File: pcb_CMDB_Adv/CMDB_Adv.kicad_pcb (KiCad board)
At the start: 6 copper layers, 59.7 x 78 mm, 9 parts, among them J1 POWER TERMINAL, J12 CONN_USB3_A, J13 CONN_USB_PWR_OTG, J15 CONN_DOCK, J16 CONN_CAM1, J17 CONN_CAM0, J2 Bus_M.2_Socket_M, J4 J_PSU_EN

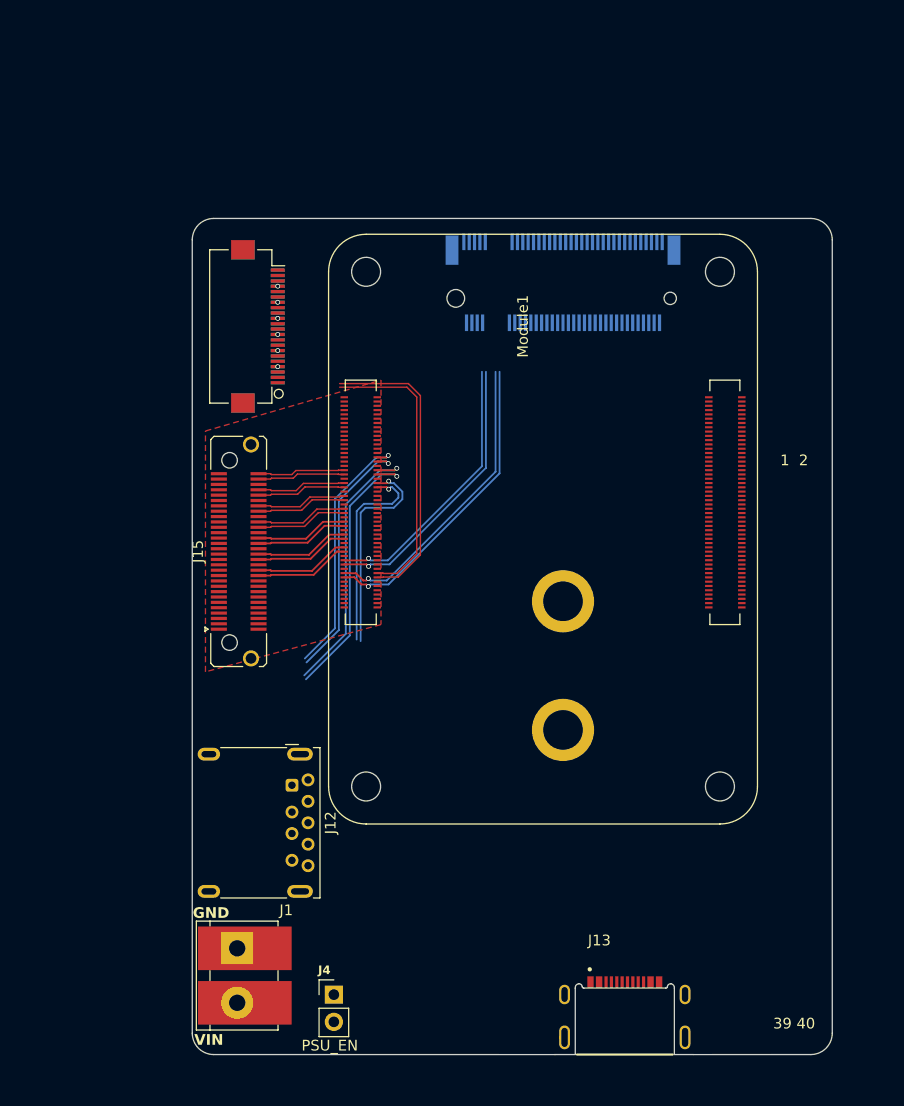
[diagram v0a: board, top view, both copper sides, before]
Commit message: CMDB-Adv PCB WIP
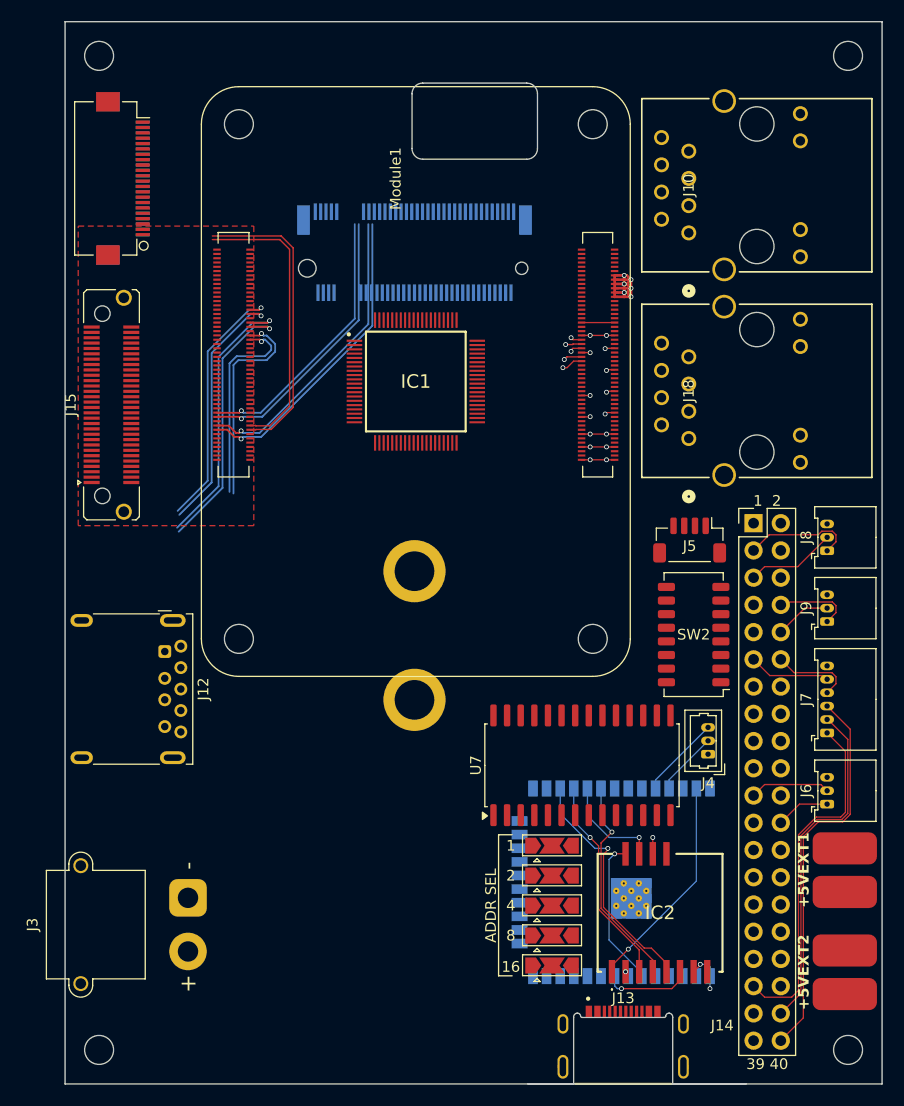
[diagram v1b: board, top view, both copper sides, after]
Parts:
- removed J1: POWER TERMINAL, CMDB_Adv:Power Terminal
- added H1: MountingHole, CMDB_Adv:MountingHole_2.7mm_M2.5_DIN965, F.Cu at (137.6, 53.4)
- added H2: MountingHole, CMDB_Adv:MountingHole_2.7mm_M2.5_DIN965, F.Cu at (207.4, 53.4)
- added H3: MountingHole, CMDB_Adv:MountingHole_2.7mm_M2.5_DIN965, F.Cu at (207.4, 146.1)
- added H4: MountingHole, CMDB_Adv:MountingHole_2.7mm_M2.5_DIN965, F.Cu at (137.6, 146.1)
- added IC1: KSZ8795CLXCC, CMDB_Adv:QFP40P1200X1200X160-80N, F.Cu at (167.1, 83.7)
- added IC2: Wio-SX1262, CMDB_Adv:Wio-SX1262, F.Cu at (189.9, 133.3)
- added J10: ETH1, CMDB_Adv:CONN12_ARJM11B1-009-AB-EW2_ABR, F.Cu at (198.9, 65.4)
- added J14: CONN_HAT, Connector_PinHeader_2.54mm:PinHeader_2x20_P2.54mm_Vertical, F.Cu at (198.6, 96.9)
- added J18: ETH2, CMDB_Adv:CONN12_ARJM11B1-009-AB-EW2_ABR, F.Cu at (198.9, 84.6)
- added J20: CONN_5VEXT1, Connector_Wire:SolderWirePad_1x01_SMD_3x6mm, F.Cu at (207.1, 131.3)
- added J21: CONN_5VEXT1_GND, Connector_Wire:SolderWirePad_1x01_SMD_3x6mm, F.Cu at (207.1, 127.3)
- added J22: CONN_5VEXT2, Connector_Wire:SolderWirePad_1x01_SMD_3x6mm, F.Cu at (207.1, 140.9)
- added J23: CONN_5VEXT2_GND, Connector_Wire:SolderWirePad_1x01_SMD_3x6mm, F.Cu at (207.1, 136.8)
- added J3: CONN_VIN, Connector_AMASS:AMASS_XT30PW-M_1x02_P2.50mm_Horizontal, F.Cu at (145.9, 131.9)
- added J5: CONN_FAN, Connector_JST:JST_SH_BM04B-SRSS-TB_1x04-1MP_P1.00mm_Vertical, F.Cu at (192.7, 98.5)
- added J6: CONN_UART3, Connector_Molex:Molex_PicoBlade_53048-0310_1x03_P1.25mm_Horizontal, F.Cu at (205.5, 123.1)
- added J7: CONN_SPI, Connector_Molex:Molex_PicoBlade_53048-0610_1x06_P1.25mm_Horizontal, F.Cu at (205.5, 116.5)
- added J8: CONN_I2C, Connector_Molex:Molex_PicoBlade_53048-0310_1x03_P1.25mm_Horizontal, F.Cu at (205.5, 99.5)
- added J9: CONN_UART0, Connector_Molex:Molex_PicoBlade_53048-0310_1x03_P1.25mm_Horizontal, F.Cu at (205.5, 106.1)
- added JP10: ADDR16, Jumper:SolderJumper-3_P2.0mm_Open_TrianglePad1.0x1.5mm, F.Cu at (179.8, 138.2)
- added JP6: ADDR1, Jumper:SolderJumper-3_P2.0mm_Open_TrianglePad1.0x1.5mm, F.Cu at (179.8, 127.0)
- added JP7: ADDR2, Jumper:SolderJumper-3_P2.0mm_Open_TrianglePad1.0x1.5mm, F.Cu at (179.8, 129.8)
- added JP8: ADDR4, Jumper:SolderJumper-3_P2.0mm_Open_TrianglePad1.0x1.5mm, F.Cu at (179.8, 132.6)
- added JP9: ADDR8, Jumper:SolderJumper-3_P2.0mm_Open_TrianglePad1.0x1.5mm, F.Cu at (179.8, 135.4)
- added SW2: SW_CONFIG, Button_Switch_SMD:SW_DIP_SPSTx08_Slide_Copal_CHS-08A_W5.08mm_P1.27mm_JPin, F.Cu at (193.0, 107.3)
- added U5: ESP32-WROOM-32UE, RF_Module:ESP32-WROOM-32UE, B.Cu at (186.2, 130.4)
- added U7: MCP23017_SO, Package_SO:SOIC-28W_7.5x17.9mm_P1.27mm, F.Cu at (182.6, 119.5)
- J4: value J_PSU_EN -> J_ESP_DBG_UART; footprint Connector_PinHeader_2.54mm:PinHeader_1x02_P2.54mm_Vertical -> Connector_Molex:Molex_PicoBlade_53047-0310_1x03_P1.25mm_Vertical
- moved J4 41.5 mm to (194.4, 118.5), turned to 90 degrees
- moved J16 18.7 mm to (139.8, 64.8)
- moved J17 18.7 mm to (139.8, 64.8)
- moved Module1 18.2 mm to (183.6, 59.7)
- moved J15 18.1 mm to (138.8, 85.9)
- moved J12 17.2 mm to (143.7, 108.9)
- moved J2 14.1 mm to (167.0, 73.2)
- moved J13 2.74 mm to (186.5, 147.6)
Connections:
- net /CM5/+5v renamed /+5VPB
- net /CM5/VBAT renamed /CM5/+3V3STB
- net /M2_3V3 renamed /+3V3PB1
- J13 pad A6: /Connectors/USBC.D_P -> /CM5/USBC.D_P
- J13 pad A7: /Connectors/USBC.D_N -> /CM5/USBC.D_N
- J13 pad B6: /Connectors/USBC.D_P -> /CM5/USBC.D_P
- J13 pad B7: /Connectors/USBC.D_N -> /CM5/USBC.D_N
- J15 pad 1: /Connectors/+3.3v -> /Connectors/+5V
- J15 pad 10: unconnected-(J15-Pin_10-Pad10) -> GND
- J15 pad 3: /Connectors/+5v -> /Connectors/+5V
- J15 pad 4: unconnected-(J15-Pin_4-Pad4) -> /CM5/+3V3RPi
- J15 pad 5: unconnected-(J15-Pin_5-Pad5) -> /Connectors/+VBUS_USBA
- J15 pad 7: unconnected-(J15-Pin_7-Pad7) -> /Connectors/+VBUS_USBA
- J15 pad 9: unconnected-(J15-Pin_9-Pad9) -> GND
- J16 pad 22: /Connectors/+3.3v -> /CM5/+3V3RPi
- J17 pad 22: /Connectors/+3.3v -> /CM5/+3V3RPi
- J4 pad 1: /PSU/VIN -> GND
- J4 pad 2: /PSU/PSU_EN -> /Platform Controller/DBG_UART_TX
- Module1 pad 11: GND -> /CM5/ETH0.P2_P
- Module1 pad 35: GND -> /CM5/GPIO1_RAW
- Module1 pad 36: GND -> /CM5/GPIO0_RAW
- Module1 pad 4: GND -> /CM5/ETH0.P1_P
- Module1 pad 41: GND -> /CM5/GP.25
- Module1 pad 51: /CM5/GPIO15_RAW -> /CM5/GP.15
- Module1 pad 55: /CM5/GPIO14_RAW -> /CM5/GP.14
- Module1 pad 6: GND -> /CM5/ETH0.P1_N
- Module1 pad 62: GND -> /CM5/CMD
- Module1 pad 78: /CM5/+3.3v_RPi -> /CM5/+3V3RPi
- Module1 pad 84: /CM5/+3.3v_RPi -> /CM5/+3V3RPi
- Module1 pad 86: /CM5/+3.3v_RPi -> /CM5/+3V3RPi
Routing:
- net /CM5/GP.17: track 0.00 -> 50.2 mm, vias 0 -> 1
- net /CM5/GP.3: track 0.00 -> 44.5 mm, vias 0 -> 1
- net /CM5/GP.2: track 0.00 -> 43.5 mm, vias 0 -> 1
- net /Connectors/GP.27: track 0.00 -> 42.3 mm
- net /CM5/GP.22: track 0.00 -> 41.7 mm
- net /CM5/GP.4: track 0.00 -> 37.0 mm, vias 0 -> 1
- net /CM5/GP.21: track 0.00 -> 36.1 mm
- net /CM5/GP.19: track 0.00 -> 32.7 mm
- net /CM5/GP.20: track 0.00 -> 32.2 mm
- net GND: track 0.00 -> 26.7 mm, vias 6 -> 18
- net /Platform Controller/LORA_RESET: track 0.00 -> 22.6 mm, vias 0 -> 1
- net /Platform Controller/LORA_RF_SW: track 0.00 -> 20.4 mm, vias 0 -> 1
- net /Platform Controller/SPI.SCLK: track 0.00 -> 19.9 mm, vias 0 -> 1
- net /Platform Controller/SPI.MOSI: track 0.00 -> 19.6 mm, vias 0 -> 1
- net /+5VPB: track 0.00 -> 16.4 mm, vias 0 -> 6
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- added copper zone on F.Cu, net /CM5/ETH0.P1_P
- removed copper zone on F.Cu, net GND
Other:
- board size 59.7 x 78 mm -> 76.2 x 99.1 mm
- board text added: "+5VEXT1"
- board text added: "+5VEXT2"
- board text added: "1"
- board text added: "16"
- board text added: "2"
- board text added: "4"
- board text added: "8"
- board text added: "ADDR SEL"
- board text removed: "PSU_EN"
- board text removed: "VIN"
